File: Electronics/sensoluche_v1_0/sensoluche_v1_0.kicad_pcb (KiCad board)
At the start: 2 copper layers, 55.1 x 57.9 mm, 25 parts, among them J1 EXT_IO_AN, J2 TB_2, P1 FSR402_Pressure

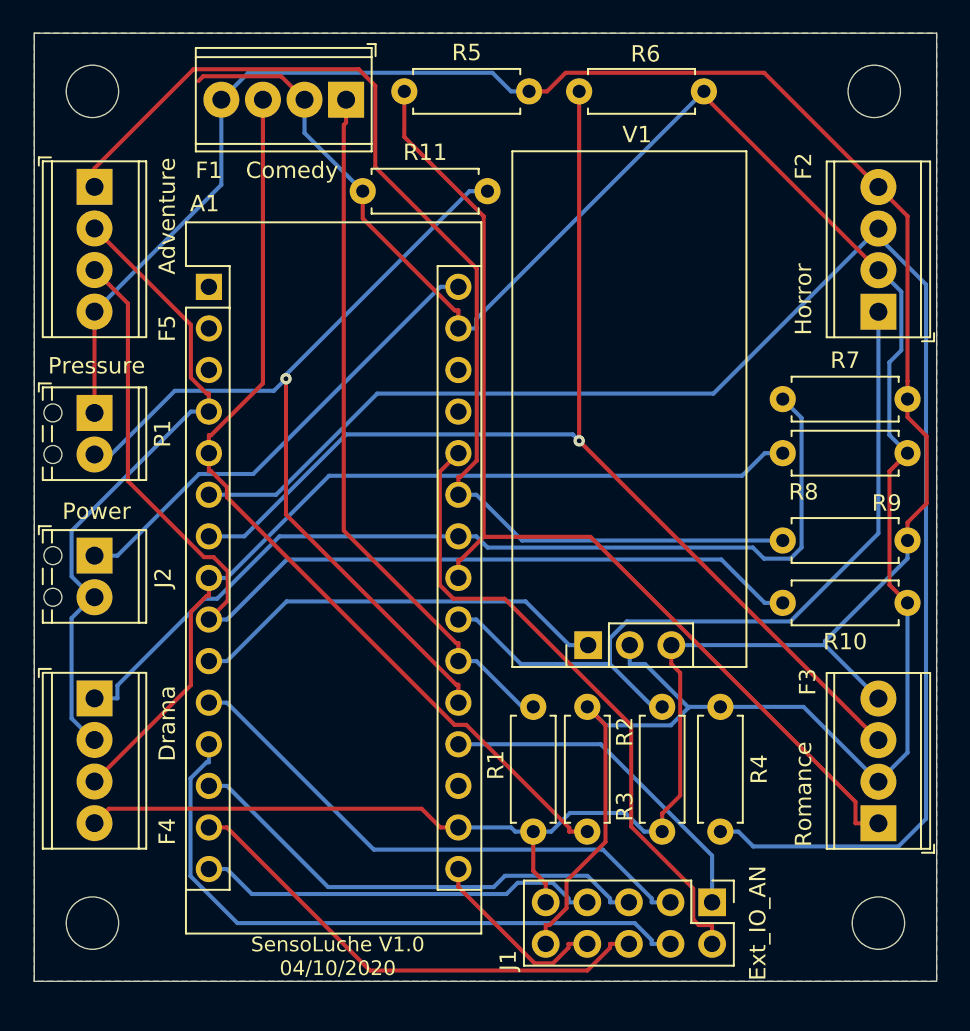
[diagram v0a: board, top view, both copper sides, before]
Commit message: V1.0 New flex sensors
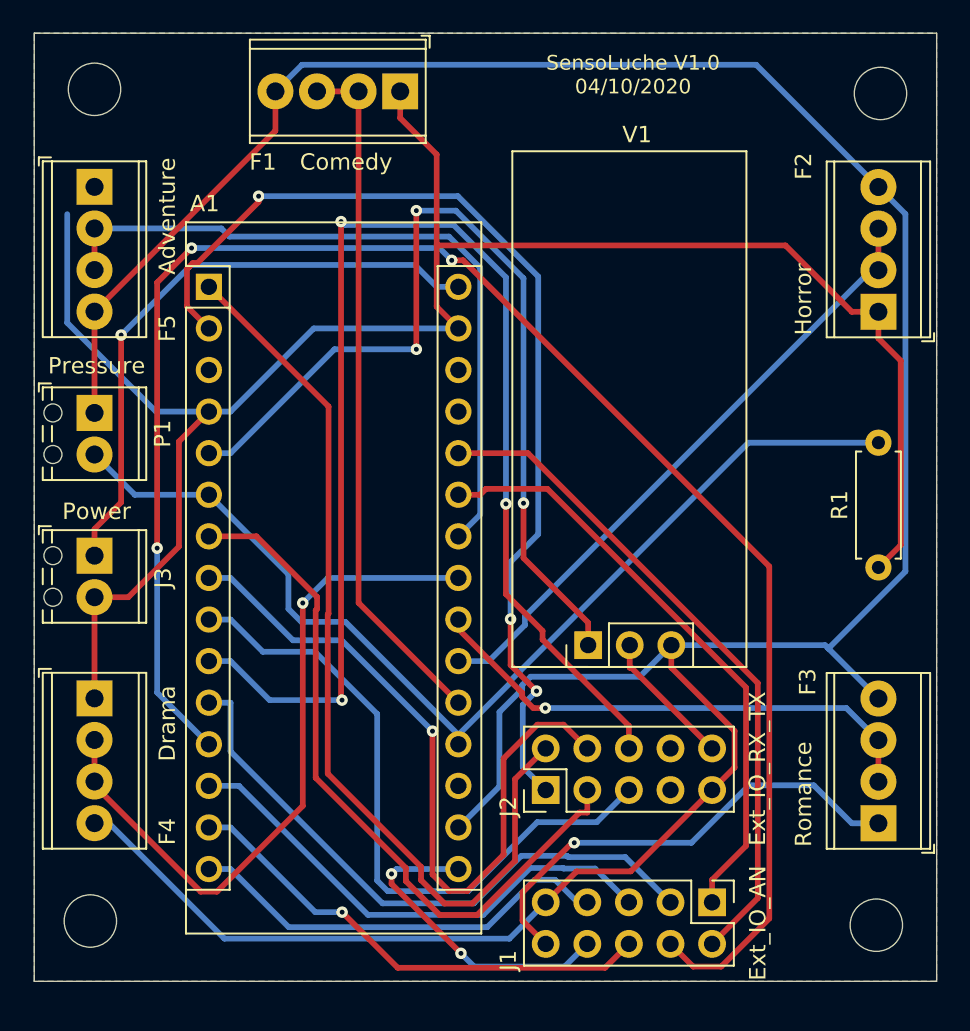
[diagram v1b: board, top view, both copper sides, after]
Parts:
- removed H_LB, H_LT, H_RB, H_RT: MountingHole_3.2mm_M3, MountingHole:MountingHole_3.2mm_M3
- removed the R1 at (151.1, 110.5)
- removed R10, R2, R4, R6, R8: 100K, Resistor_THT:R_Axial_DIN0207_L6.3mm_D2.5mm_P7.62mm_Horizontal
- removed R3, R5, R7, R9: 22K, Resistor_THT:R_Axial_DIN0207_L6.3mm_D2.5mm_P7.62mm_Horizontal
- added BOTTOM_LEFT_HOLE: MountingHole_3.2mm_M3, MountingHole:MountingHole_3.2mm_M3, F.Cu at (124.1, 123.6)
- added BOTTOM_RIGTH_HOLE: MountingHole_3.2mm_M3, MountingHole:MountingHole_3.2mm_M3, F.Cu at (172.1, 123.8)
- added J2: EXT_IO_AN, Connector_PinHeader_2.54mm:PinHeader_2x05_P2.54mm_Vertical, F.Cu at (151.9, 115.6)
- added TOP_LEFT_HOLE: MountingHole_3.2mm_M3, MountingHole:MountingHole_3.2mm_M3, F.Cu at (124.3, 72.8)
- added TOP_RIGTH_HOLE: MountingHole_3.2mm_M3, MountingHole:MountingHole_3.2mm_M3, F.Cu at (172.3, 73.0)
- moved R1 39.0 mm to (172.2, 102.0), turned to 90 degrees
- moved F1 3.34 mm to (143.0, 72.9)
- renumbered J2 to J3, R11 to R1
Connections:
- A1 pad 1: Net-(A1-Pad1) -> /D1_TX
- A1 pad 10: /D_Vibration -> /D7
- A1 pad 19: /A0 -> /A_Pressure
- A1 pad 2: Net-(A1-Pad2) -> /D0_RX
- A1 pad 20: /A_Pressure -> /A_Comedy
- A1 pad 21: /A_Comedy -> /A_Horror
- A1 pad 22: /A_Horror -> /A_Romance
- A1 pad 23: /A_Romance -> /A_Drama
- A1 pad 24: /A_Drama -> /A_Adventure
- A1 pad 25: /A_Adventure -> /A6
- A1 pad 5: /D_Comedy -> /D_Vibration
- A1 pad 6: /D_Horror -> /A_Pressure
- A1 pad 7: /D_Romance -> /D4
- A1 pad 8: /D_Drama -> /D5
- A1 pad 9: /D_Adventure -> /D6
- F1 pad 1: /A_Comedy -> GND
- F1 pad 2: GND -> /A_Comedy
- F1 pad 3: /D_Comedy -> /A_Comedy
- F2 pad 1: /A_Horror -> GND
- F2 pad 2: GND -> /A_Horror
- F2 pad 3: /D_Horror -> /A_Horror
- F3 pad 1: /A_Romance -> GND
- F3 pad 2: GND -> /A_Romance
- F3 pad 3: /D_Romance -> /A_Romance
- F4 pad 1: /A_Drama -> GND
- F4 pad 2: GND -> /A_Drama
- F4 pad 3: /D_Drama -> /A_Drama
- F5 pad 1: /A_Adventure -> GND
- F5 pad 2: GND -> /A_Adventure
- F5 pad 3: /D_Adventure -> /A_Adventure
- J1 pad 1: /A0 -> /A6
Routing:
- net /D_Horror: track 98.4 -> 0.00 mm
- net /D7: track 0.00 -> 81.7 mm, vias 0 -> 3
- net /D_Romance: track 72.6 -> 0.00 mm, vias 1 -> 0
- net /D9: track 39.8 -> 105.2 mm, vias 0 -> 3
- net /D0_RX: track 0.00 -> 63.4 mm, vias 0 -> 3
- net /D_Adventure: track 63.2 -> 0.00 mm
- net /D_Comedy: track 56.9 -> 0.00 mm
- net /D1_TX: track 0.00 -> 56.7 mm
- net /D_Drama: track 53.6 -> 0.00 mm
- net /D5: track 0.00 -> 44.4 mm, vias 0 -> 1
- net /D4: track 0.00 -> 43.7 mm
- net /D6: track 0.00 -> 41.0 mm
- net /A6: track 0.00 -> 36.7 mm
- net /A_Romance: track 64.6 -> 31.7 mm, vias 0 -> 1
- net /D_Vibration: track 25.8 -> 56.1 mm, vias 0 -> 3
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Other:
- net class Default: clearance 0.175 -> 0.35; trace_width 0.25 -> 0.35
- rule trace_clearance: 0.175 -> 0.35
- board text added: "Ext_IO_RX_TX"
